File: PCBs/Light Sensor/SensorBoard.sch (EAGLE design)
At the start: 12 parts, among them J1 AVR_SPI_PRG_6PTH

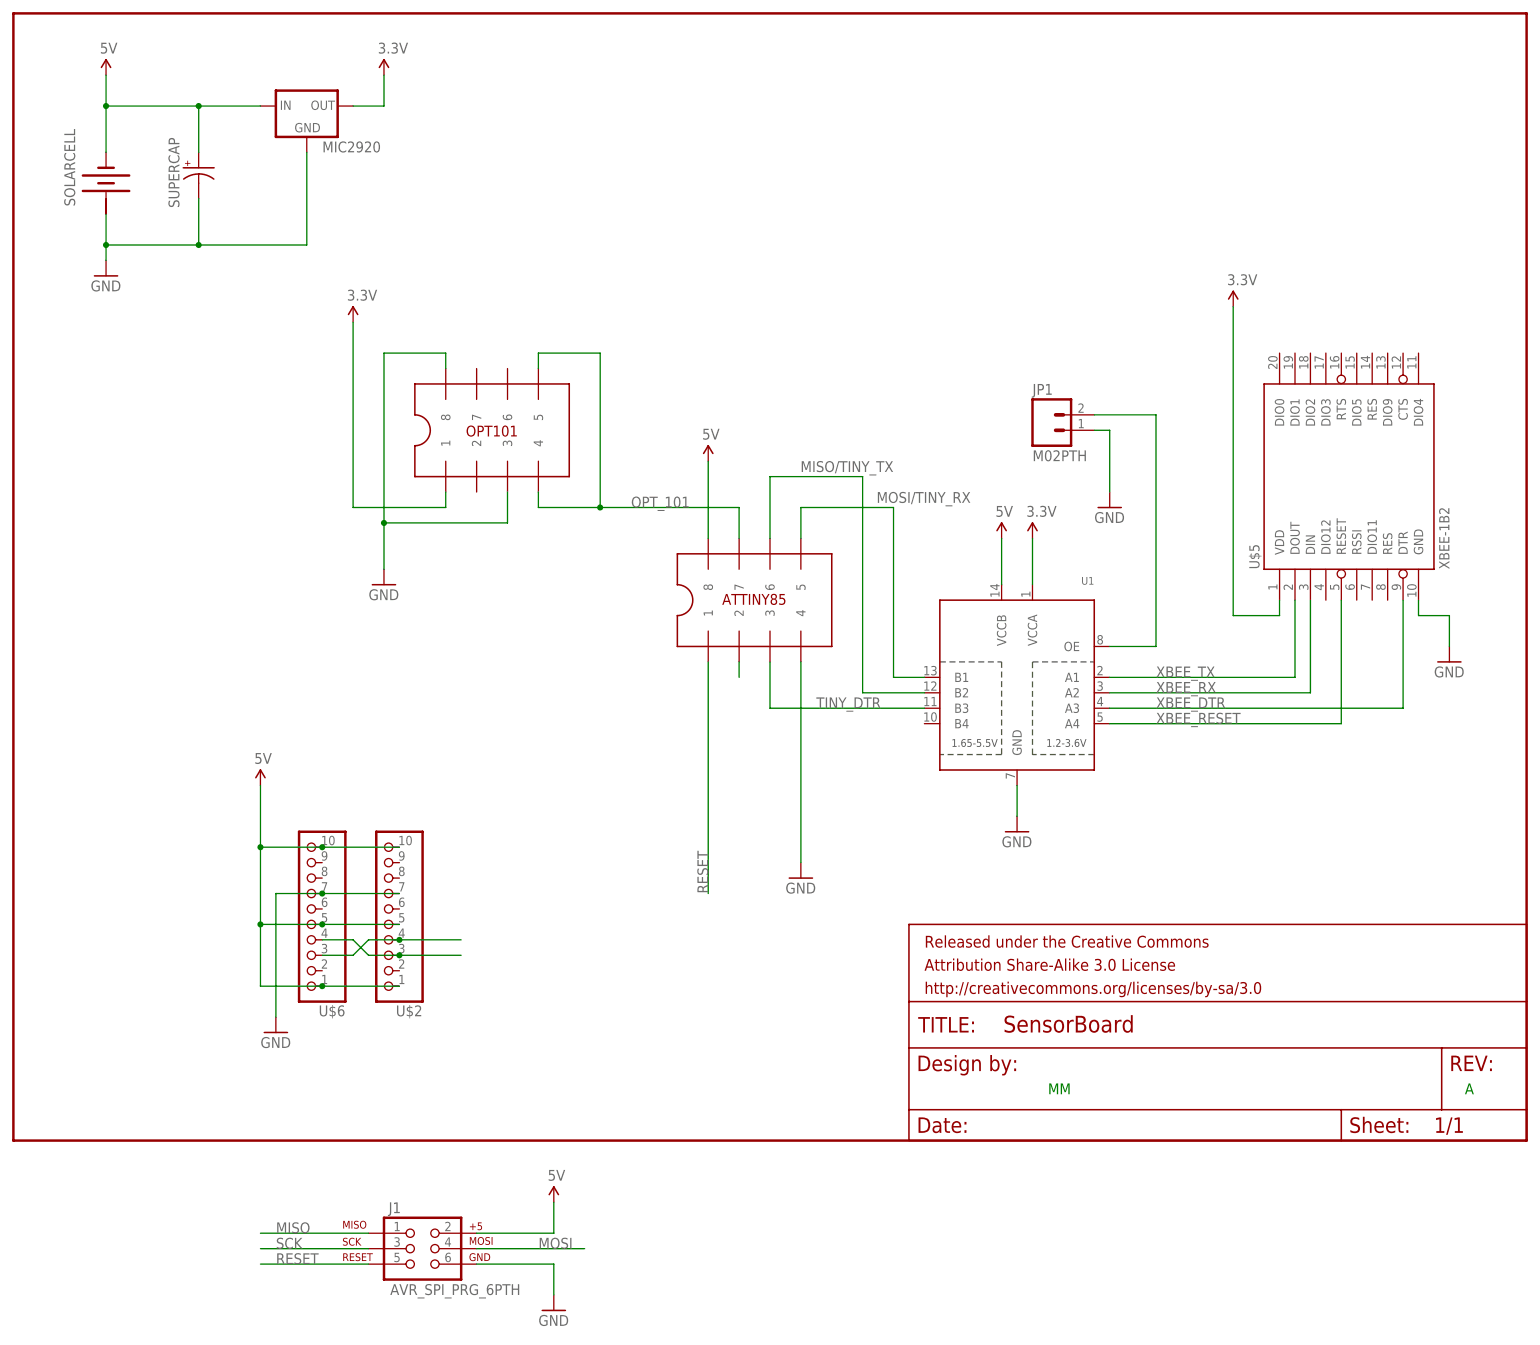
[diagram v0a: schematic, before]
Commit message: Cleanups
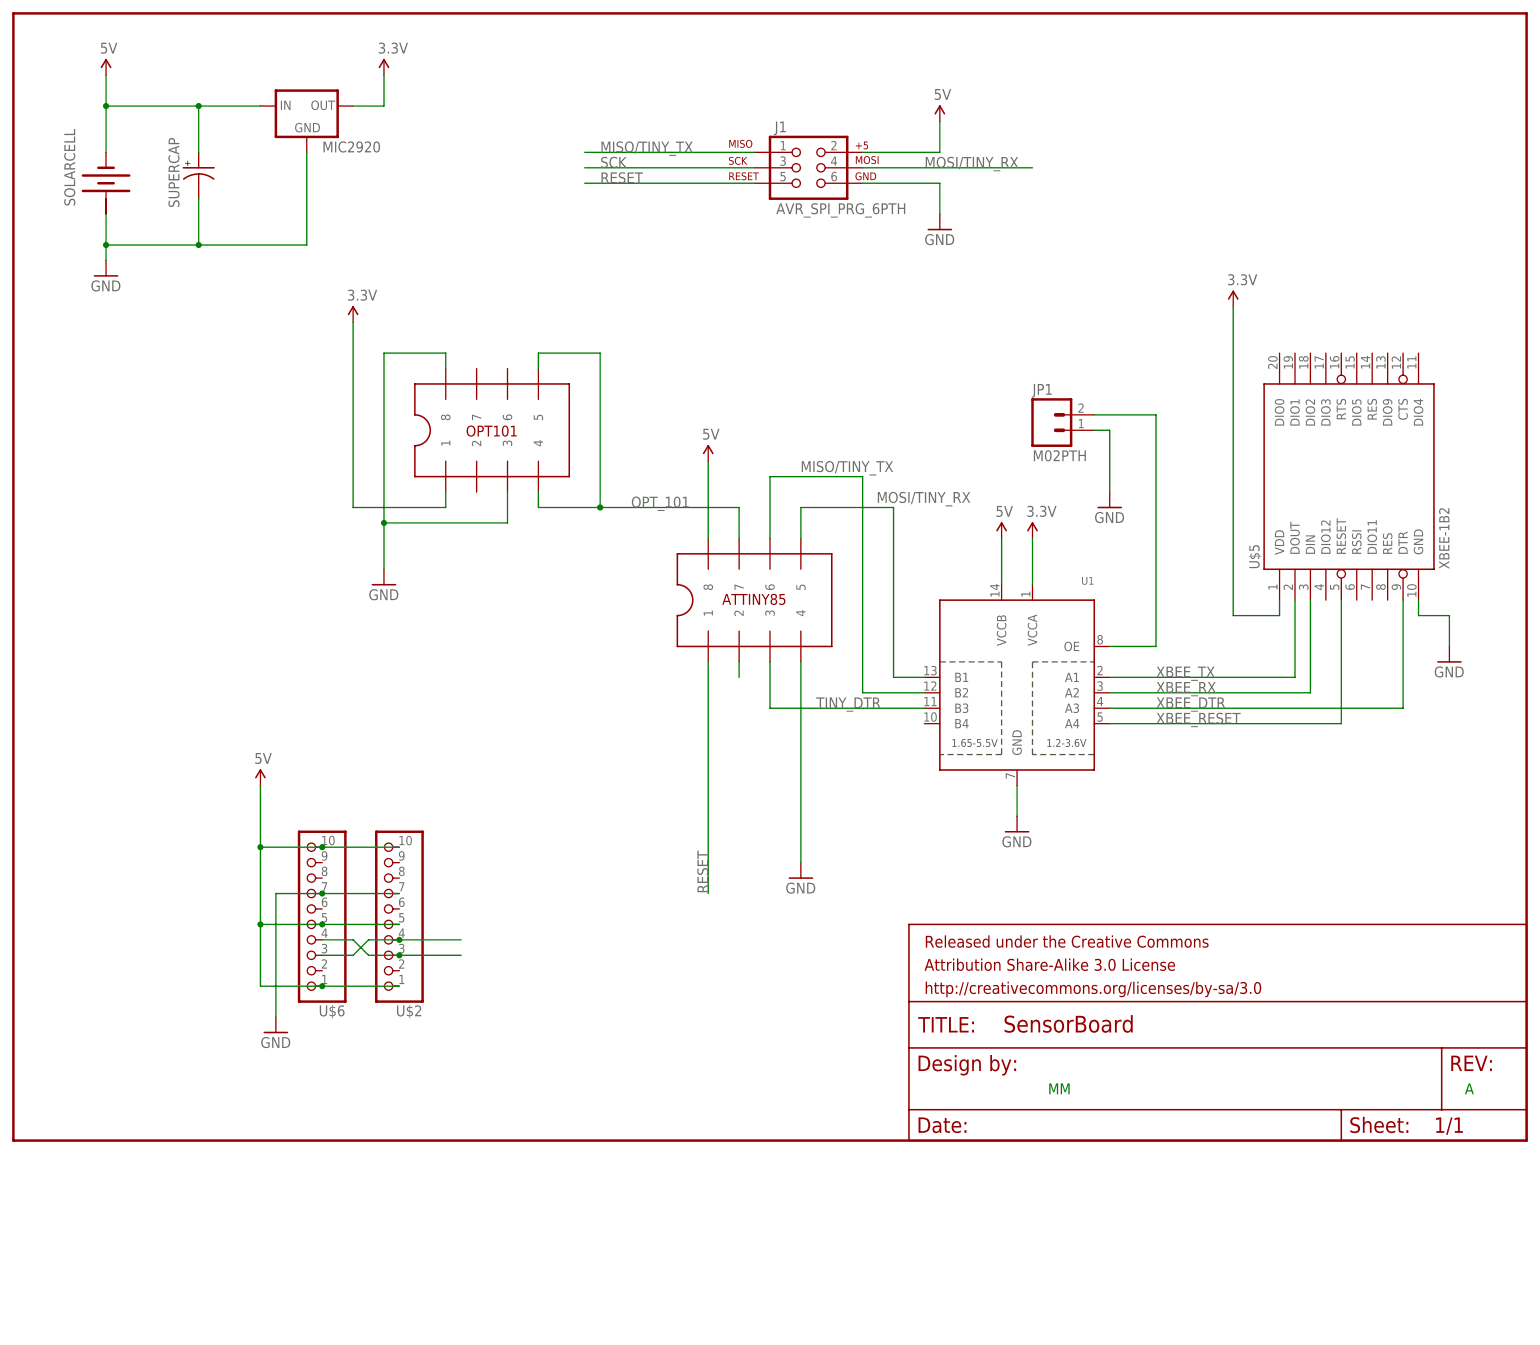
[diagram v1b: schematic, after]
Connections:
- removed net MISO: J1.1
- removed net MOSI: J1.4
- net MISO/TINY_TX: now also J1.1
- net MOSI/TINY_RX: now also J1.4
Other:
- moved on the sheet: J1
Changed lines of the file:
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@@
 <instance part="FRAME1" gate="G$1" x="0" y="0"/>
 <instance part="FRAME1" gate="G$2" x="147.32" y="0"/>
-<instance part="J1" gate="G$1" x="66.04" y="-17.78"/>
-<instance part="SUPPLY4" gate="G$1" x="88.9" y="-10.16"/>
+<instance part="J1" gate="G$1" x="129.54" y="160.02"/>
+<instance part="SUPPLY4" gate="G$1" x="152.4" y="167.64"/>
 <instance part="GND1" gate="1" x="15.24" y="142.24"/>
 <instance part="GND2" gate="1" x="60.96" y="91.44"/>
-<instance part="GND3" gate="1" x="88.9" y="-27.94"/>
+<instance part="GND3" gate="1" x="152.4" y="149.86"/>
 <instance part="GND4" gate="1" x="129.54" y="43.18"/>
 <instance part="GND5" gate="1" x="236.22" y="78.74"/>
@@
 <segment>
 <pinref part="J1" gate="G$1" pin="2"/>
-<wire x1="76.2" y1="-15.24" x2="88.9" y2="-15.24" width="0.1524" layer="91"/>
+<wire x1="139.7" y1="162.56" x2="152.4" y2="162.56" width="0.1524" layer="91"/>
 <pinref part="SUPPLY4" gate="G$1" pin="5V"/>
-<wire x1="88.9" y1="-10.16" x2="88.9" y2="-15.24" width="0.1524" layer="91"/>
+<wire x1="152.4" y1="167.64" x2="152.4" y2="162.56" width="0.1524" layer="91"/>
 </segment>
 <segment>
@@
 <segment>
 <pinref part="J1" gate="G$1" pin="3"/>
-<wire x1="58.42" y1="-17.78" x2="40.64" y2="-17.78" width="0.1524" layer="91"/>
-<label x="43.18" y="-17.78" size="1.778" layer="95"/>
+<wire x1="121.92" y1="160.02" x2="93.98" y2="160.02" width="0.1524" layer="91"/>
+<label x="96.52" y="160.02" size="1.778" layer="95"/>
 </segment>
 </net>
@@
 <segment>
 <pinref part="J1" gate="G$1" pin="5"/>
-<wire x1="58.42" y1="-20.32" x2="40.64" y2="-20.32" width="0.1524" layer="91"/>
-<label x="43.18" y="-20.32" size="1.778" layer="95"/>
-</segment>
-</net>
-<net name="MISO" class="0">
-<segment>
-<pinref part="J1" gate="G$1" pin="1"/>
-<wire x1="58.42" y1="-15.24" x2="40.64" y2="-15.24" width="0.1524" layer="91"/>
-<label x="43.18" y="-15.24" size="1.778" layer="95"/>
-</segment>
-</net>
-<net name="MOSI" class="0">
-<segment>
-<pinref part="J1" gate="G$1" pin="4"/>
-<wire x1="76.2" y1="-17.78" x2="93.98" y2="-17.78" width="0.1524" layer="91"/>
-<label x="86.36" y="-17.78" size="1.778" layer="95"/>
+<wire x1="121.92" y1="157.48" x2="93.98" y2="157.48" width="0.1524" layer="91"/>
+<label x="96.52" y="157.48" size="1.778" layer="95"/>
 </segment>
 </net>
@@
 <segment>
 <pinref part="J1" gate="G$1" pin="6"/>
-<wire x1="76.2" y1="-20.32" x2="88.9" y2="-20.32" width="0.1524" layer="91"/>
-<wire x1="88.9" y1="-20.32" x2="88.9" y2="-25.4" width="0.1524" layer="91"/>
+<wire x1="139.7" y1="157.48" x2="152.4" y2="157.48" width="0.1524" layer="91"/>
+<wire x1="152.4" y1="157.48" x2="152.4" y2="152.4" width="0.1524" layer="91"/>
 <pinref part="GND3" gate="1" pin="GND"/>
 </segment>
@@
 <wire x1="144.78" y1="76.2" x2="149.86" y2="76.2" width="0.1524" layer="91"/>
 </segment>
+<segment>
+<pinref part="J1" gate="G$1" pin="4"/>
+<wire x1="139.7" y1="160.02" x2="167.64" y2="160.02" width="0.1524" layer="91"/>
+<label x="149.86" y="160.02" size="1.778" layer="95"/>
+</segment>
 </net>
 <net name="MISO/TINY_TX" class="0">
@@
 <wire x1="139.7" y1="73.66" x2="149.86" y2="73.66" width="0.1524" layer="91"/>
 </segment>
-</net>
+<segment>
+<pinref part="J1" gate="G$1" pin="1"/>
+<wire x1="121.92" y1="162.56" x2="93.98" y2="162.56" width="0.1524" layer="91"/>
+<label x="96.52" y="162.56" size="1.778" layer="95"/>
+</segment>
+</net>
